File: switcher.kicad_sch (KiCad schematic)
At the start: 0 parts

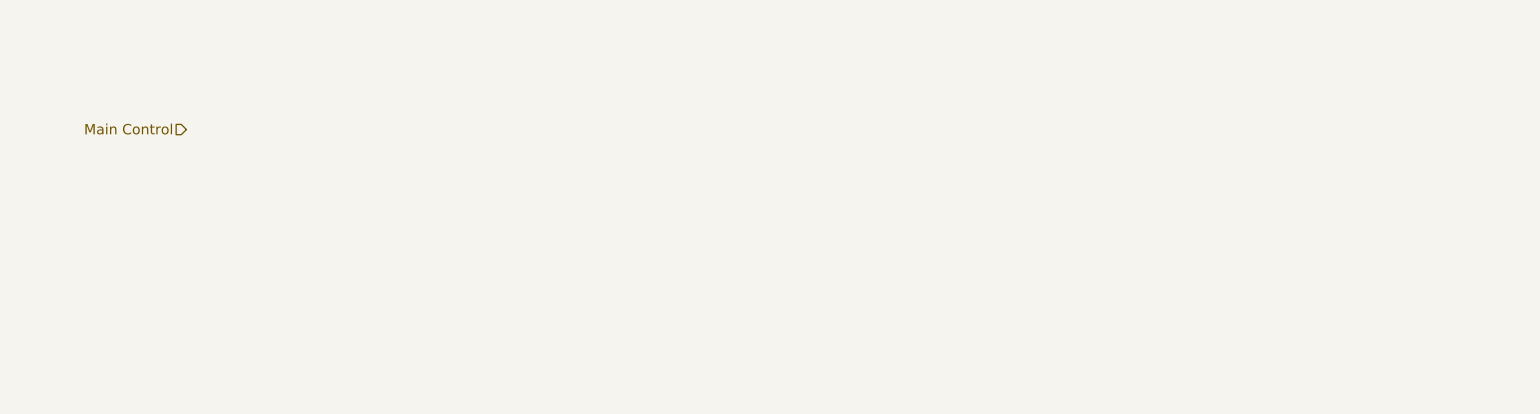
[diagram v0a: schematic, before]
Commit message: Finished basic version
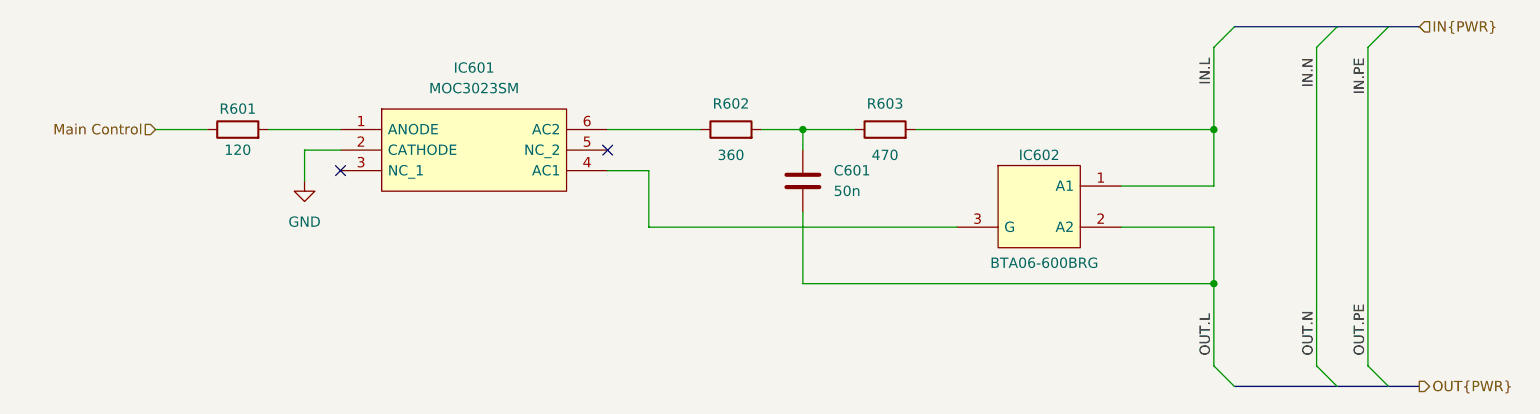
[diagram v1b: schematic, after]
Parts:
- added C601: 50n, symbol Device:C
- added IC601: MOC3023SM, MOC3043SM, symbol OxySwitch:MOC3023SM
- added IC602: BTA06-600BRG, TO255P460X1020X2005-3P, symbol OxySwitch:BTA06-600BRG
- added R601: 120, symbol Device:R
- added R602: 360, symbol Device:R
- added R603: 470, symbol Device:R
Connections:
- net Main Control: now also R601.1
- new net: IC601.1 (ANODE), R601.2
- new net: IC601.4 (AC1), IC602.3 (G)
- new net: IC601.6 (AC2), R602.1
- new net: C601.1, R602.2, R603.1
- new net GND: IC601.2 (CATHODE)
- new net IN.L: IC602.1 (A1), R603.2
- new net OUT.L: C601.2, IC602.2 (A2)
- no-connect marks 0 -> 2
